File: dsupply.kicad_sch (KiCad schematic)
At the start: 61 parts, among them J5 Barrel_Jack, Q2 BSS138, Q3 BSS138, Q4 BC857, Q5 AOSP21321, Q6 BC857, U21 ACPL-217-500E, U22 TPS54620, U24 PM1202, U25 AMS1117-3.3

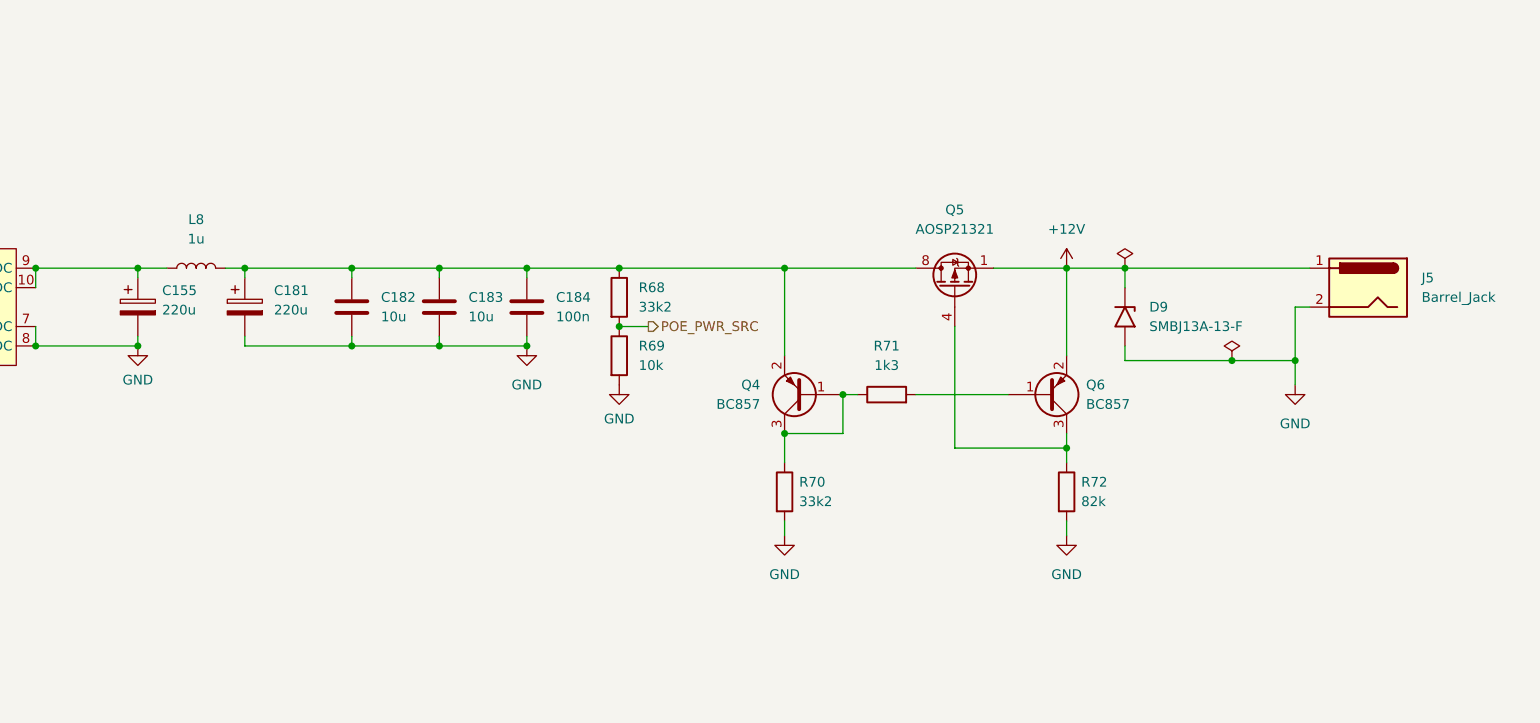
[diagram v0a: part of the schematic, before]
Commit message: sync
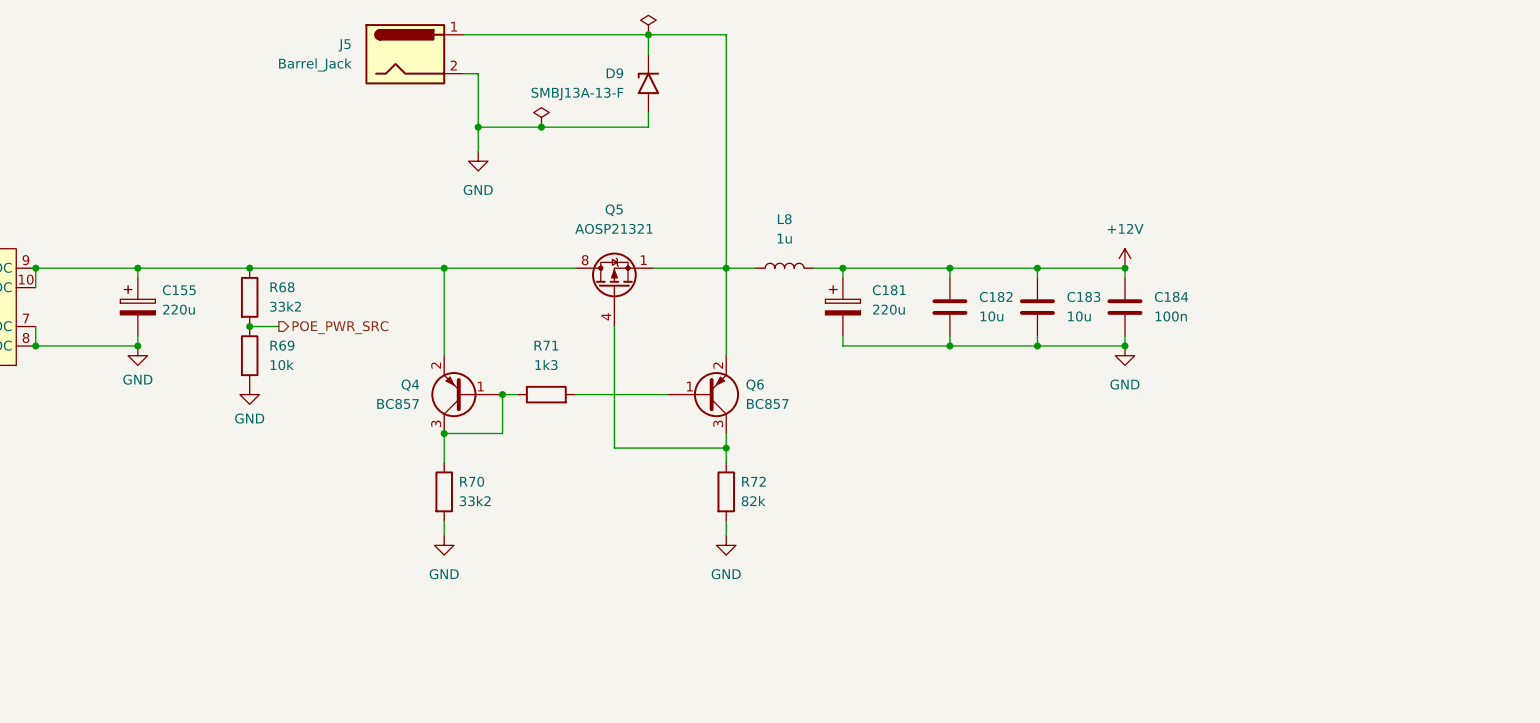
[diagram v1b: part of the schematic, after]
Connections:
- net +12V: now also C181.1, C182.1, C183.1, C184.1, L8.2; no longer D9.1 (A1), J5.1, Q5.1 (S), Q5.2 (S), Q5.3 (S), Q6.2 (E)
- net at Q4.2 (E), Q5.5 (D), Q5.6 (D)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: now also C155.1, U24.10 (+VDC), U24.9 (+VDC); no longer C181.1, C182.1, C183.1, C184.1, L8.2
- new net: D9.1 (A1), J5.1, L8.1, Q5.1 (S), Q5.2 (S), Q5.3 (S), Q6.2 (E)
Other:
- moved on the sheet: C181, C182, C183, C184, D9, J5, L8, Q4, Q5, Q6, R68, R69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
